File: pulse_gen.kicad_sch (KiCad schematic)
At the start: 13 parts, among them Q1 NPN, Q2 NPN, U3 ${SIM.PARAMS}

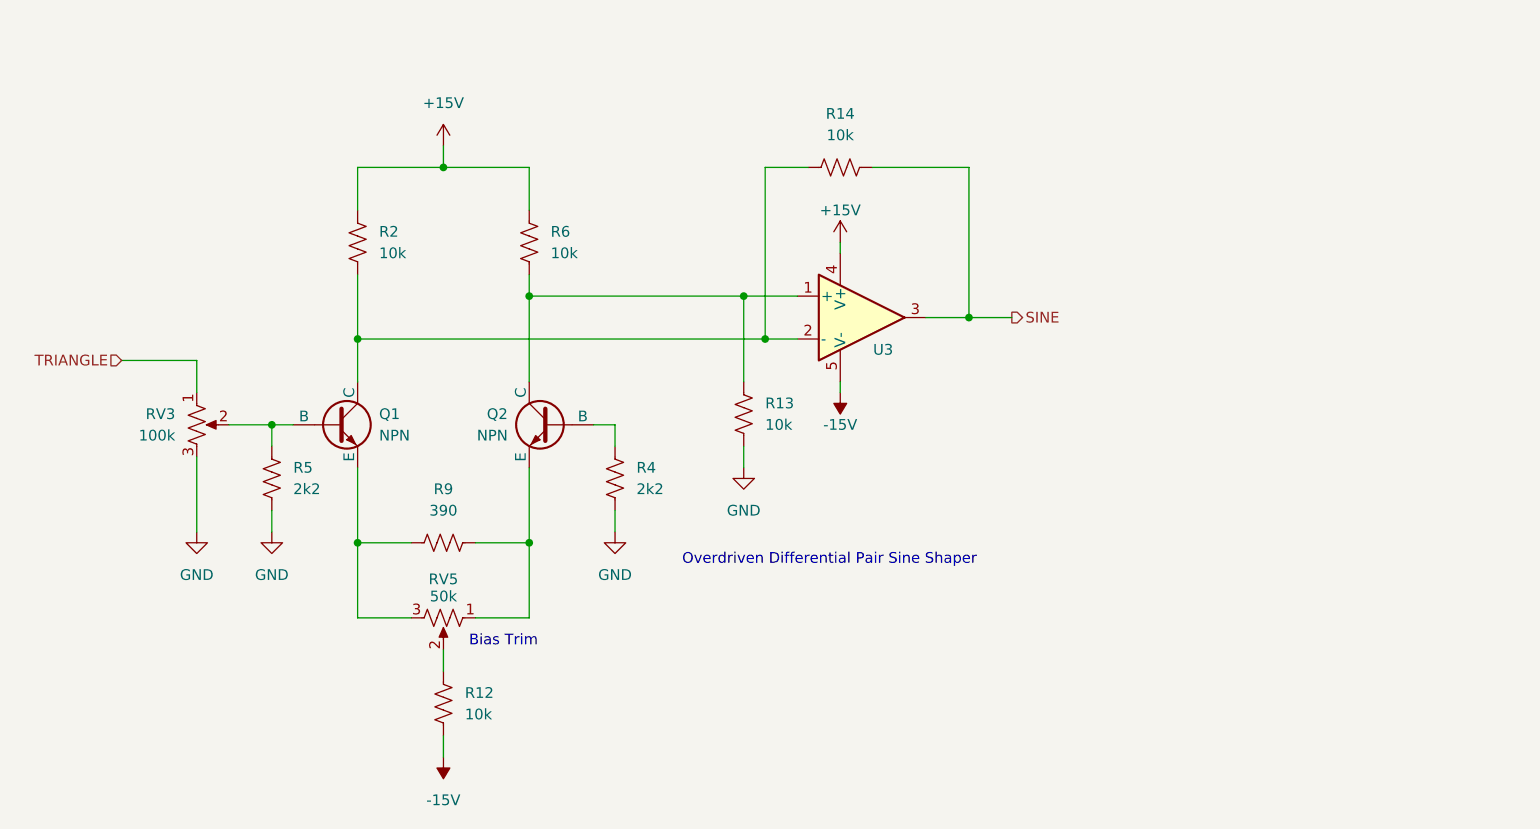
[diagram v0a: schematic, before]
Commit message: added pulse gen and other stuff
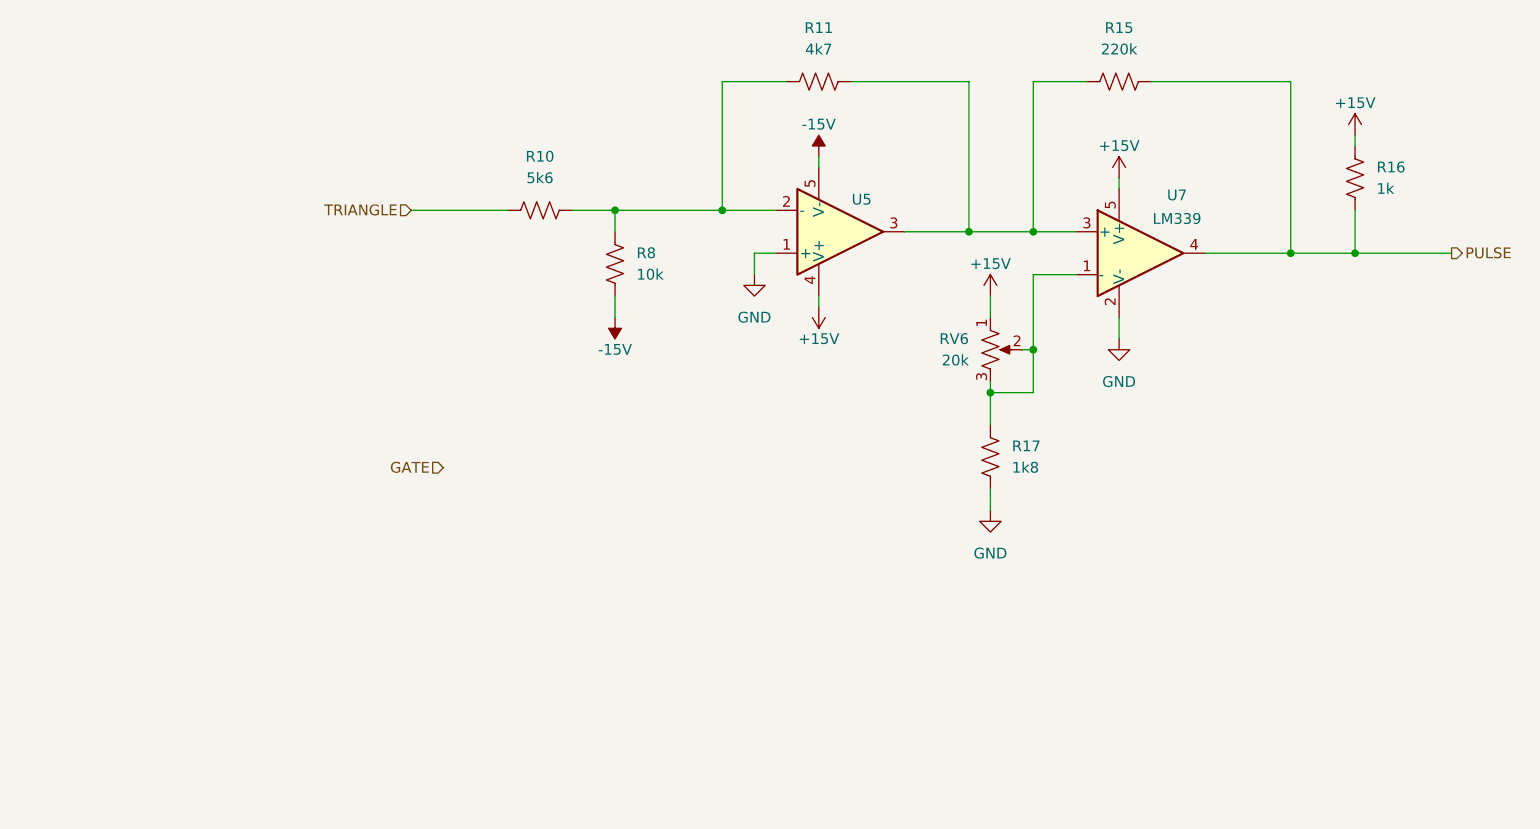
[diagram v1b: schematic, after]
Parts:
- removed Q1, Q2: NPN, symbol Simulation_SPICE:NPN
- removed R12, R13, R14, R2, R6: 10k, symbol Device:R_US
- removed R4, R5: 2k2, symbol Device:R_US
- removed R9: 390, symbol Device:R_US
- removed RV3: 100k, symbol Device:R_Potentiometer_US
- removed RV5: 50k, symbol Device:R_Potentiometer_US
- removed U3: ${SIM.PARAMS}, symbol Simulation_SPICE:OPAMP
- added R10: 5k6, symbol Device:R_US
- added R11: 4k7, symbol Device:R_US
- added R15: 220k, symbol Device:R_US
- added R16: 1k, symbol Device:R_US
- added R17: 1k8, symbol Device:R_US
- added R8: 10k, symbol Device:R_US
- added RV6: 20k, symbol Device:R_Potentiometer_US
- added U5: ${SIM.PARAMS}, symbol Simulation_SPICE:OPAMP
- added U7: LM339, Package_TO_SOT_SMD:SOT-23-5, symbol Comparator:LM397
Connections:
- net +15V: now also R16.2, RV6.1, U5.4 (V+), U7.5 (V+)
- net -15V: now also R8.2, U5.5 (V-)
- net GND: now also R17.2, U5.1 (+), U7.2 (V-)
- net TRIANGLE: now also R10.1
- new net: R11.2, R15.1, U5.3, U7.3 (+)
- new net: R10.2, R11.1, R8.1, U5.2 (-)
- new net: R17.1, RV6.2, RV6.3, U7.1 (-)
- new net PULSE: R15.2, R16.1, U7.4
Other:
- note removed: "Bias Trim"
- note removed: "Overdriven Differential Pair Sine Shaper"
